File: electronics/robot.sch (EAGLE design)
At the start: 67 parts, among them J1 USB-B, J2 DC21MMX, J3 B6B-ZR, J4 B6B-ZR, J5 B6B-ZR, J6 KICKER, Q1 IRLMS2002TRPBF, Q2 IRLMS2002TRPBF, Q3 NPN_BC817,215, Q4 SUD50N04-8M8P-4GE3, Q5 NPN_BC817,215, Q6 NPN_BC817,215, U1 FT232L, U2 ESP32-WROOM-32E_(16MB), U3 S8252, U4 L9110, U5 L9110, U6 L9110, U7 MT3608

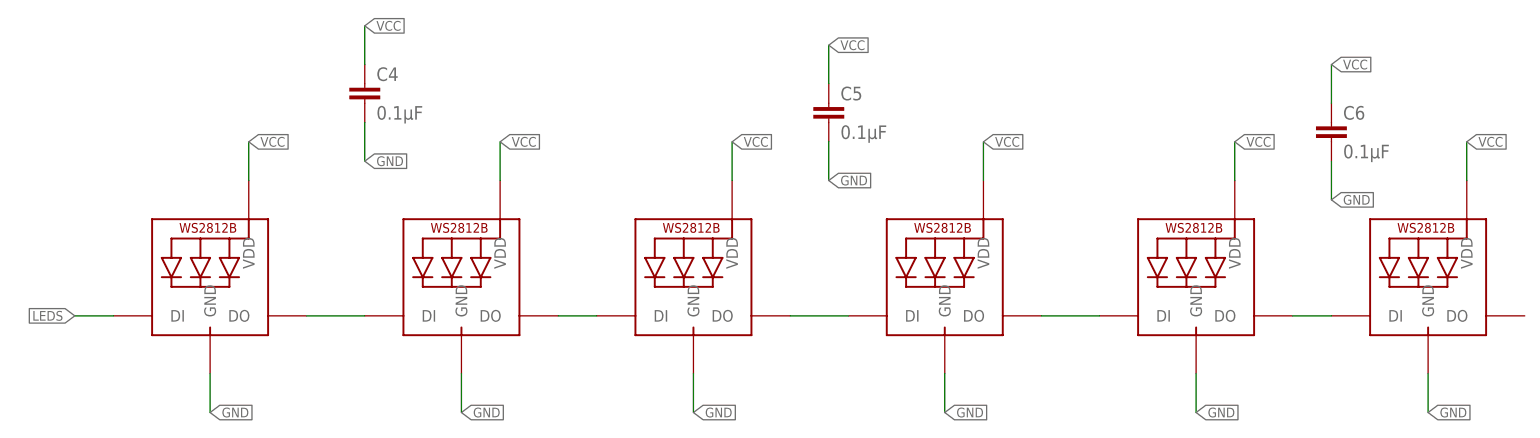
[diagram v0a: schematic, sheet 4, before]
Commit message: rev0
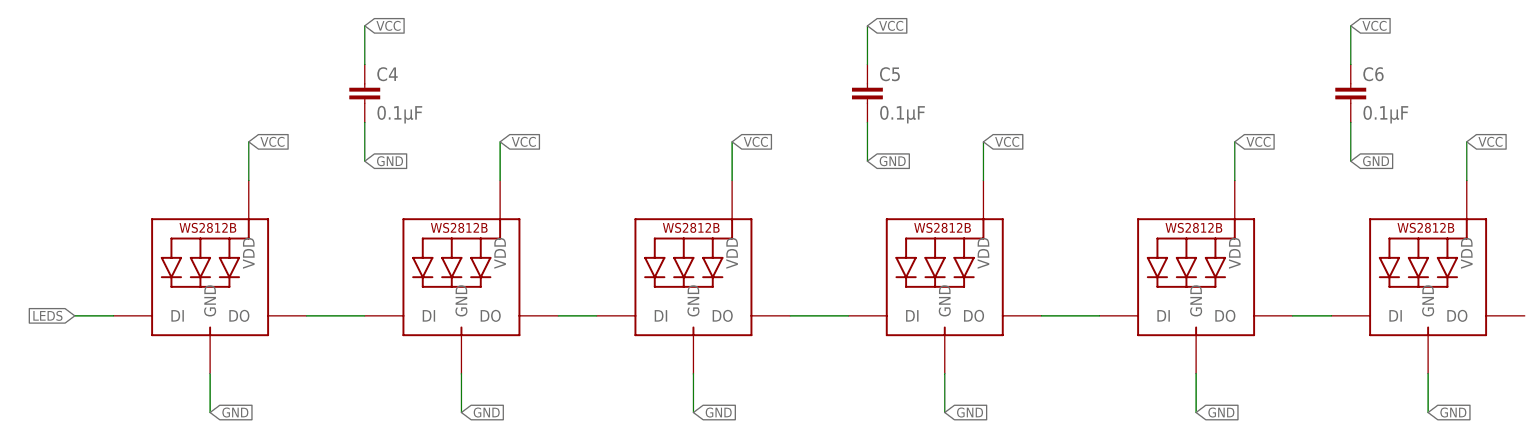
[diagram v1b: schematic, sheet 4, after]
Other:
- moved on the sheet: C5, C6
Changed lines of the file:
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@@
 <attribute name="FARNELL" x="-55.88" y="22.86" size="1.778" layer="96" display="off"/>
 </instance>
-<instance part="C5" gate="G$1" x="5.08" y="20.32">
-<attribute name="FARNELL" x="5.08" y="20.32" size="1.778" layer="96" display="off"/>
+<instance part="C5" gate="G$1" x="10.16" y="22.86">
+<attribute name="FARNELL" x="10.16" y="22.86" size="1.778" layer="96" display="off"/>
 </instance>
-<instance part="C6" gate="G$1" x="71.12" y="17.78">
-<attribute name="FARNELL" x="71.12" y="17.78" size="1.778" layer="96" display="off"/>
+<instance part="C6" gate="G$1" x="73.66" y="22.86">
+<attribute name="FARNELL" x="73.66" y="22.86" size="1.778" layer="96" display="off"/>
 </instance>
 </instances>
@@
 </segment>
 <segment>
-<wire x1="5.08" y1="17.78" x2="5.08" y2="12.7" width="0.1524" layer="91"/>
-<label x="5.08" y="12.7" size="1.27" layer="95" xref="yes"/>
+<wire x1="10.16" y1="20.32" x2="10.16" y2="15.24" width="0.1524" layer="91"/>
+<label x="10.16" y="15.24" size="1.27" layer="95" xref="yes"/>
 <pinref part="C5" gate="G$1" pin="2"/>
 </segment>
 <segment>
-<wire x1="71.12" y1="15.24" x2="71.12" y2="10.16" width="0.1524" layer="91"/>
-<label x="71.12" y="10.16" size="1.27" layer="95" xref="yes"/>
+<wire x1="73.66" y1="20.32" x2="73.66" y2="15.24" width="0.1524" layer="91"/>
+<label x="73.66" y="15.24" size="1.27" layer="95" xref="yes"/>
 <pinref part="C6" gate="G$1" pin="2"/>
 </segment>
@@
 </segment>
 <segment>
-<wire x1="5.08" y1="25.4" x2="5.08" y2="30.48" width="0.1524" layer="91"/>
-<label x="5.08" y="30.48" size="1.27" layer="95" xref="yes"/>
+<wire x1="10.16" y1="27.94" x2="10.16" y2="33.02" width="0.1524" layer="91"/>
+<label x="10.16" y="33.02" size="1.27" layer="95" xref="yes"/>
 <pinref part="C5" gate="G$1" pin="1"/>
 </segment>
@@
 </segment>
 <segment>
-<wire x1="71.12" y1="22.86" x2="71.12" y2="27.94" width="0.1524" layer="91"/>
-<label x="71.12" y="27.94" size="1.27" layer="95" xref="yes"/>
+<wire x1="73.66" y1="27.94" x2="73.66" y2="33.02" width="0.1524" layer="91"/>
+<label x="73.66" y="33.02" size="1.27" layer="95" xref="yes"/>
 <pinref part="C6" gate="G$1" pin="1"/>
 </segment>

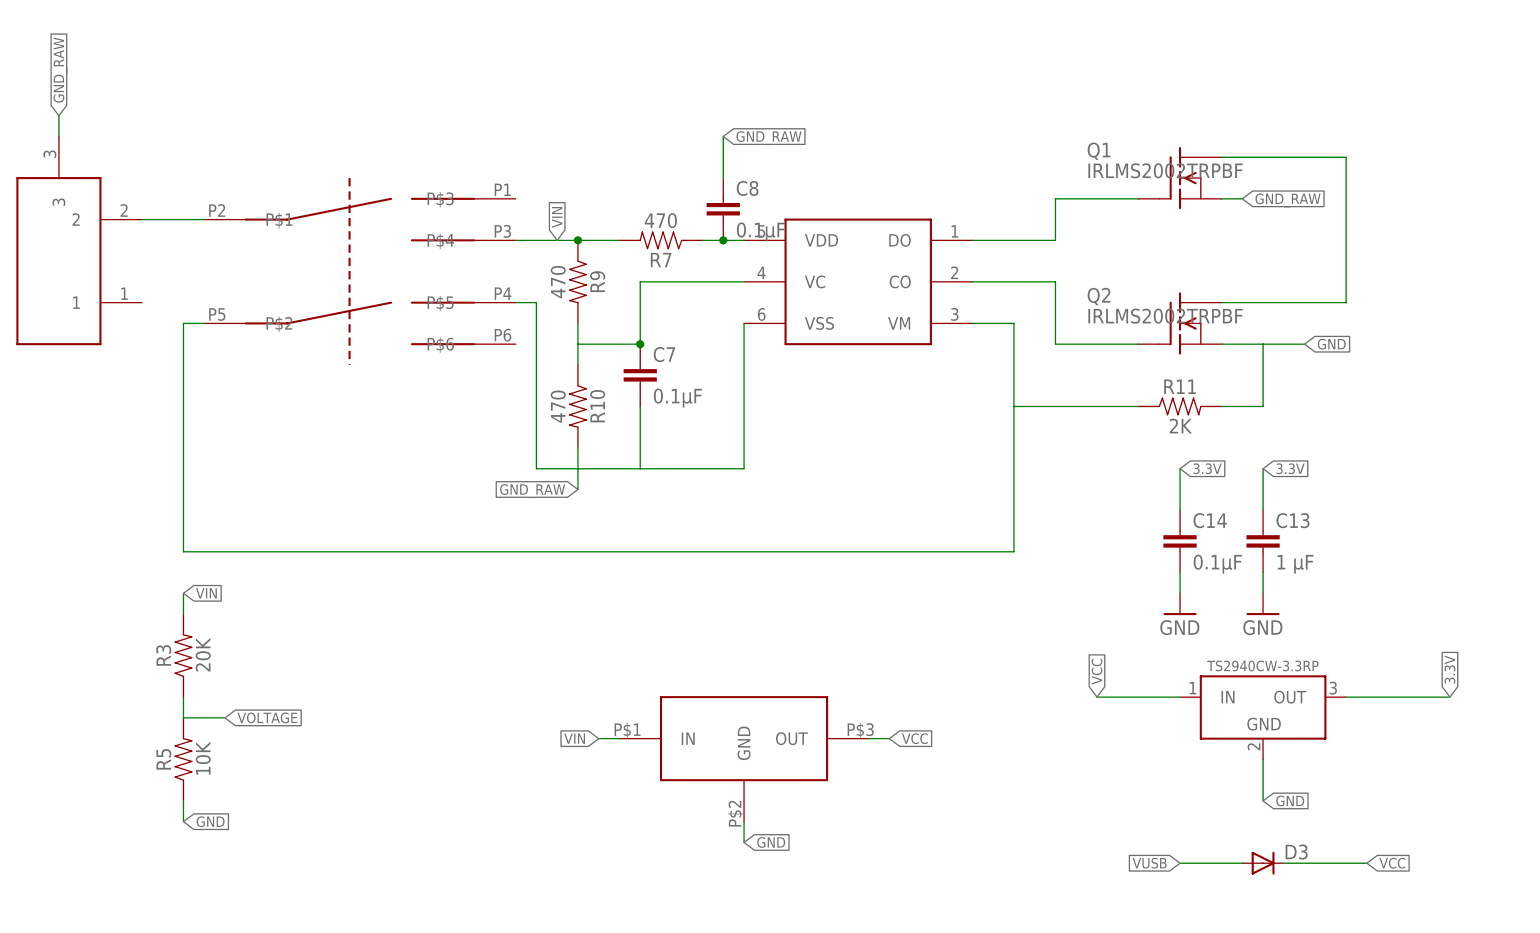
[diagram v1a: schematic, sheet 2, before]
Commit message: Electronic fixes
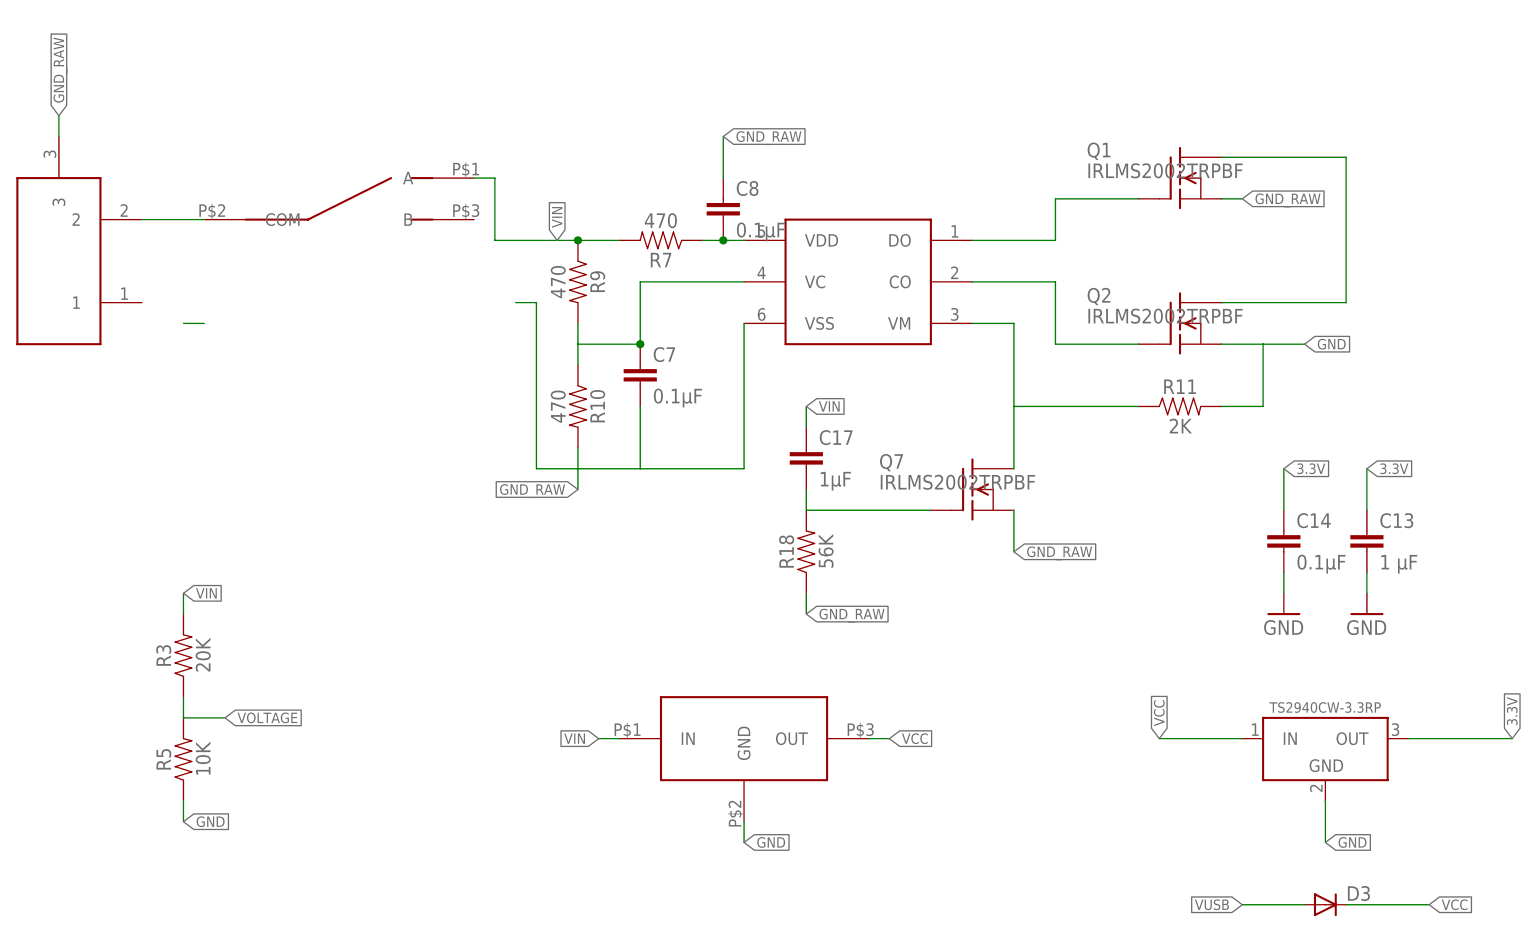
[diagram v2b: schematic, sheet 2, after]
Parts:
- removed S1: DPDT, rhoban:DPDT
- added C17: 1µF, SparkFun-Capacitors:0.33UF/330NF-0805-50V-10%
- added Q7: IRLMS2002TRPBF, rhoban:IRLMS2002TRPBF
- added R18: 56K, SparkFun-Resistors:0.3OHM-0805-1/8W-1%
- added U$1: L102011ML04Q, rhoban:L102011ML04Q
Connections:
- new net N$19: C17.2, Q7.G, R18.2
- net GND_RAW: now also Q7.S, R18.1; no longer S1.P$5
- net N$13: now also Q7.D; no longer S1.P$2
- net N$7: now also U$1.COM; no longer S1.P$1
- net VIN: now also C17.1, U$1.A; no longer S1.P$4
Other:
- moved on the sheet: C13, C14, D3
